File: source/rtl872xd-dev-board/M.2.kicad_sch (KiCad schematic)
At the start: 1 part, among them J2 Bus_M.2_Socket_B

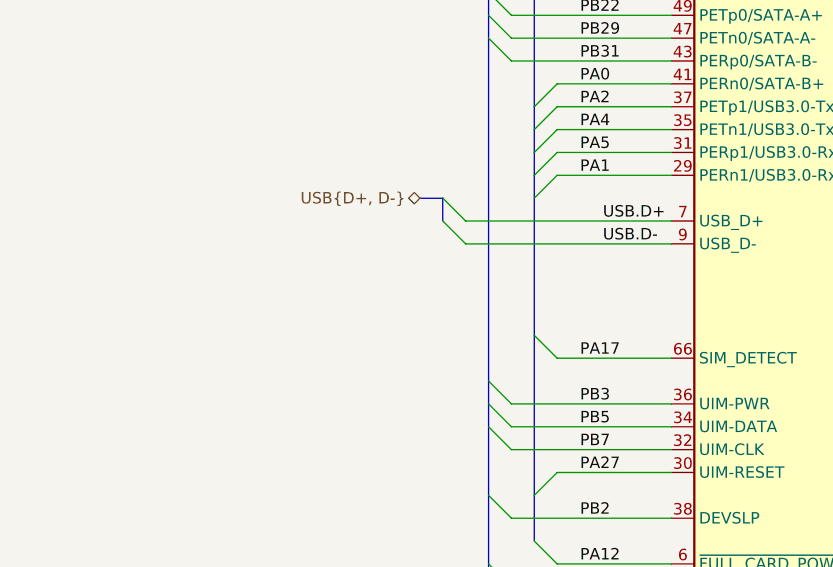
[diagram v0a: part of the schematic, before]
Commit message: first production version
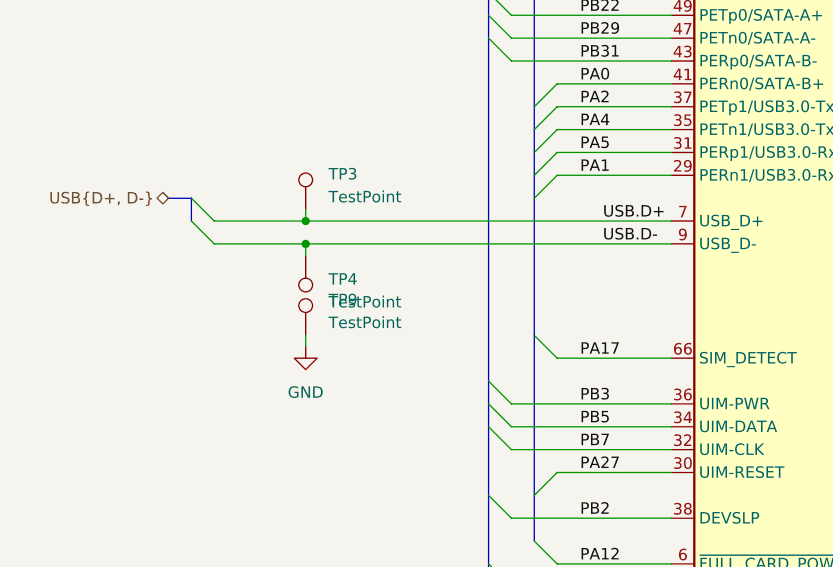
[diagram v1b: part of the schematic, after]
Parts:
- added TP3, TP4, TP9: TestPoint, TestPoint:TestPoint_Pad_D1.0mm, symbol Connector:TestPoint
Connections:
- net GND: now also TP9.1
- net USB.D+: now also TP3.1
- net USB.D-: now also TP4.1
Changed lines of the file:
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@@
   (junction (at 116.84 152.4) (diameter 0) (color 0 0 0 0)
   )
+  (junction (at 50.8 91.44) (diameter 0) (color 0 0 0 0)
+  )
   (junction (at 116.84 50.8) (diameter 0) (color 0 0 0 0)
   )
@@
   (junction (at 71.12 40.64) (diameter 0) (color 0 0 0 0)
   )
+  (junction (at 50.8 93.98) (diameter 0) (color 0 0 0 0)
+  )
   (bus_entry (at 154.94 58.42) (size 2.54 -2.54)
     (stroke (width 0) (type default))
   )
-  (bus_entry (at 68.58 93.98) (size -2.54 -2.54)
-    (stroke (width 0) (type default))
-  )
-  (bus_entry (at 68.58 91.44) (size -2.54 -2.54)
+  (bus_entry (at 40.64 93.98) (size -2.54 -2.54)
+    (stroke (width 0) (type default))
+  )
+  (bus_entry (at 40.64 91.44) (size -2.54 -2.54)
     (stroke (width 0) (type default))
   )
@@
     (stroke (width 0) (type default))
   )
+  (wire (pts (xy 50.8 104.14) (xy 50.8 105.41))
+    (stroke (width 0) (type default))
+  )
   (bus (pts (xy 76.2 66.04) (xy 76.2 78.74))
     (stroke (width 0) (type default))
@@
     (stroke (width 0) (type default))
   )
+  (wire (pts (xy 50.8 90.17) (xy 50.8 91.44))
+    (stroke (width 0) (type default))
+  )
   (wire (pts (xy 142.24 139.7) (xy 154.94 139.7))
     (stroke (width 0) (type default))
@@
     (stroke (width 0) (type default))
   )
+  (wire (pts (xy 50.8 93.98) (xy 91.44 93.98))
+    (stroke (width 0) (type default))
+  )
   (bus (pts (xy 71.12 111.76) (xy 71.12 114.3))
     (stroke (width 0) (type default))
@@
     (stroke (width 0) (type default))
   )
-  (bus (pts (xy 63.5 88.9) (xy 66.04 88.9))
+  (bus (pts (xy 35.56 88.9) (xy 38.1 88.9))
     (stroke (width 0) (type default))
   )
@@
     (stroke (width 0) (type default))
   )
+  (wire (pts (xy 50.8 93.98) (xy 50.8 95.25))
+    (stroke (width 0) (type default))
+  )
   (wire (pts (xy 142.24 111.76) (xy 154.94 111.76))
     (stroke (width 0) (type default))
@@
     (stroke (width 0) (type default))
   )
-  (wire (pts (xy 68.58 91.44) (xy 91.44 91.44))
+  (wire (pts (xy 40.64 91.44) (xy 50.8 91.44))
     (stroke (width 0) (type default))
   )
@@
     (stroke (width 0) (type default))
   )
-  (wire (pts (xy 68.58 93.98) (xy 91.44 93.98))
+  (wire (pts (xy 40.64 93.98) (xy 50.8 93.98))
+    (stroke (width 0) (type default))
+  )
+  (wire (pts (xy 50.8 91.44) (xy 91.44 91.44))
     (stroke (width 0) (type default))
   )
@@
     (stroke (width 0) (type default))
   )
-  (bus (pts (xy 66.04 88.9) (xy 66.04 91.44))
+  (bus (pts (xy 38.1 88.9) (xy 38.1 91.44))
     (stroke (width 0) (type default))
   )
@@
     (effects (font (size 1.27 1.27)) (justify right))
   )
-  (hierarchical_label "USB{D+, D-}" (shape bidirectional) (at 63.5 88.9 180) (fields_autoplaced)
+  (hierarchical_label "USB{D+, D-}" (shape bidirectional) (at 35.56 88.9 180) (fields_autoplaced)
     (effects (font (size 1.27 1.27)) (justify right))
+  )
+  (symbol (lib_id "power:GND") (at 50.8 105.41 0) (unit 1)
+    (in_bom yes) (on_board yes) (dnp no) (fields_autoplaced)
+    (property "Reference" "#PWR036" (at 50.8 111.76 0)
+      (effects (font (size 1.27 1.27)) hide)
+    )
+    (property "Value" "GND" (at 50.8 110.49 0)
+      (effects (font (size 1.27 1.27)))
+    )
+    (property "Footprint" "" (at 50.8 105.41 0)
+      (effects (font (size 1.27 1.27)) hide)
+    )
+    (property "Datasheet" "" (at 50.8 105.41 0)
+      (effects (font (size 1.27 1.27)) hide)
+    )
+    (pin "1")
+    (instances
+      (project "rtl872xd-dev-board"
+        (path "/5477044b-5ae5-4ed6-bb7d-f5f3cc95a2d4/bdc7329f-2717-4429-9357-eafb26421b20"
+          (reference "#PWR036") (unit 1)
+        )
+      )
+    )
   )
   (symbol (lib_id "power:GND") (at 116.84 153.67 0) (unit 1)
@@
         (path "/5477044b-5ae5-4ed6-bb7d-f5f3cc95a2d4/bdc7329f-2717-4429-9357-eafb26421b20"
           (reference "#PWR031") (unit 1)
+        )
+      )
+    )
+  )
+  (symbol (lib_id "Connector:TestPoint") (at 50.8 95.25 180) (unit 1)
+    (in_bom yes) (on_board yes) (dnp no) (fields_autoplaced)
+    (property "Reference" "TP4" (at 53.34 97.917 0)
+      (effects (font (size 1.27 1.27)) (justify right))
+    )
+    (property "Value" "TestPoint" (at 53.34 100.457 0)
+      (effects (font (size 1.27 1.27)) (justify right))
+    )
+    (property "Footprint" "TestPoint:TestPoint_Pad_D1.0mm" (at 45.72 95.25 0)
+      (effects (font (size 1.27 1.27)) hide)
+    )
+    (property "Datasheet" "~" (at 45.72 95.25 0)
+      (effects (font (size 1.27 1.27)) hide)
+    )
+    (pin "1")
+    (instances
+      (project "rtl872xd-dev-board"
+        (path "/5477044b-5ae5-4ed6-bb7d-f5f3cc95a2d4/bdc7329f-2717-4429-9357-eafb26421b20"
+          (reference "TP4") (unit 1)
         )
       )
@@
     )
   )
+  (symbol (lib_id "Connector:TestPoint") (at 50.8 90.17 0) (unit 1)
+    (in_bom yes) (on_board yes) (dnp no) (fields_autoplaced)
+    (property "Reference" "TP3" (at 53.34 86.233 0)
+      (effects (font (size 1.27 1.27)) (justify left))
+    )
+    (property "Value" "TestPoint" (at 53.34 88.773 0)
+      (effects (font (size 1.27 1.27)) (justify left))
+    )
+    (property "Footprint" "TestPoint:TestPoint_Pad_D1.0mm" (at 55.88 90.17 0)
+      (effects (font (size 1.27 1.27)) hide)
+    )
+    (property "Datasheet" "~" (at 55.88 90.17 0)
+      (effects (font (size 1.27 1.27)) hide)
+    )
+    (pin "1")
+    (instances
+      (project "rtl872xd-dev-board"
+        (path "/5477044b-5ae5-4ed6-bb7d-f5f3cc95a2d4/bdc7329f-2717-4429-9357-eafb26421b20"
+          (reference "TP3") (unit 1)
+        )
+      )
+    )
+  )
   (symbol (lib_id "power:+3.3V") (at 116.84 49.53 0) (unit 1)
     (in_bom yes) (on_board yes) (dnp no) (fields_autoplaced)
@@
         )
       )
+    )
+  )
+  (symbol (lib_id "Connector:TestPoint") (at 50.8 104.14 0) (unit 1)
+    (in_bom yes) (on_board yes) (dnp no) (fields_autoplaced)
+    (property "Reference" "TP9" (at 53.34 100.203 0)
+      (effects (font (size 1.27 1.27)) (justify left))
+    )
+    (property "Value" "TestPoint" (at 53.34 102.743 0)
+      (effects (font (size 1.27 1.27)) (justify left))
+    )
+    (property "Footprint" "TestPoint:TestPoint_Pad_D1.0mm" (at 55.88 104.14 0)
+      (effects (font (size 1.27 1.27)) hide)
+    )
+    (property "Datasheet" "~" (at 55.88 104.14 0)
+      (effects (font (size 1.27 1.27)) hide)
+    )
+    (pin "1")
+    (instances
+      (project "rtl872xd-dev-board"
+        (path "/5477044b-5ae5-4ed6-bb7d-f5f3cc95a2d4/bdc7329f-2717-4429-9357-eafb26421b20"
+          (reference "TP9") (unit 1)
+        )
+      )
